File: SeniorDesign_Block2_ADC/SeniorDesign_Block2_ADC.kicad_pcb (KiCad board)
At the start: 2 copper layers, 40 x 75 mm, 18 parts, among them J1 Conn_02x18_Row_Letter_First, J2 Conn_02x18_Row_Letter_First, U1 AD9283, X1 ASE-xxxMHz

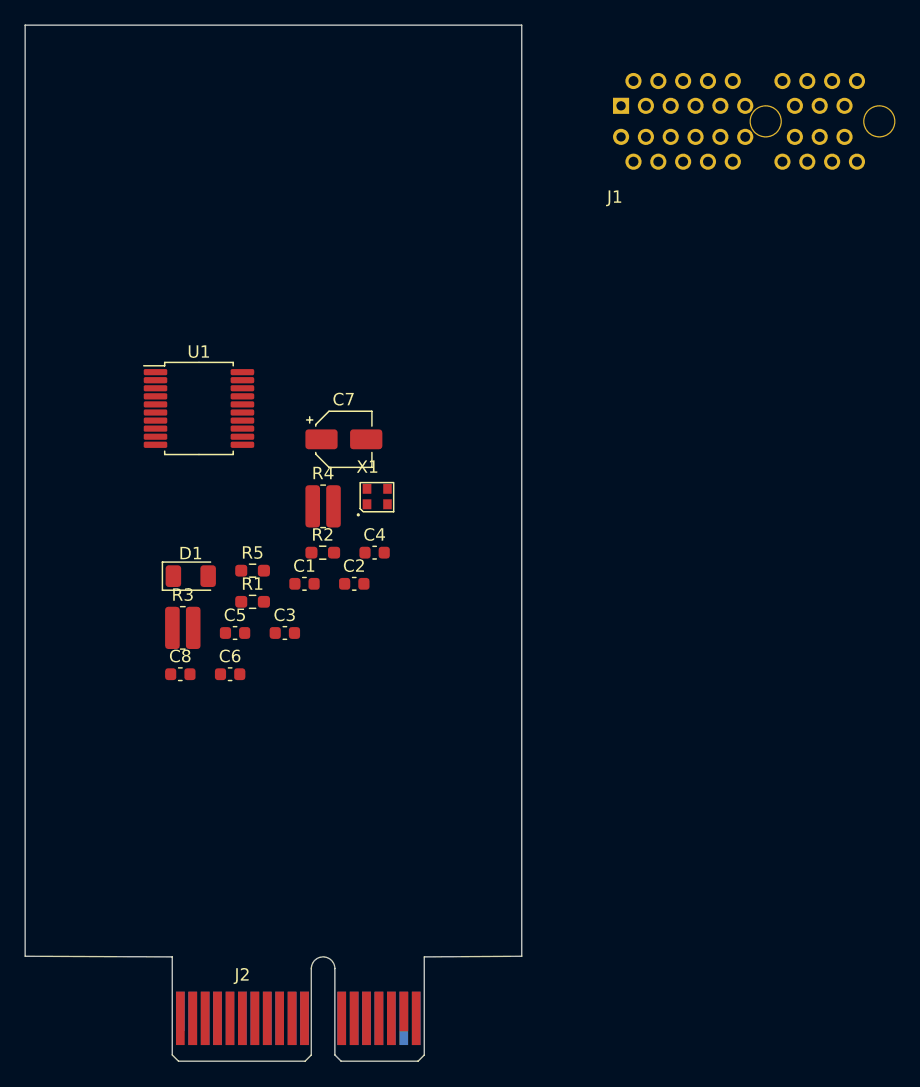
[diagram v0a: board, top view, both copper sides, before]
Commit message: Continued work.  Push to github.  Even worse commit messages.
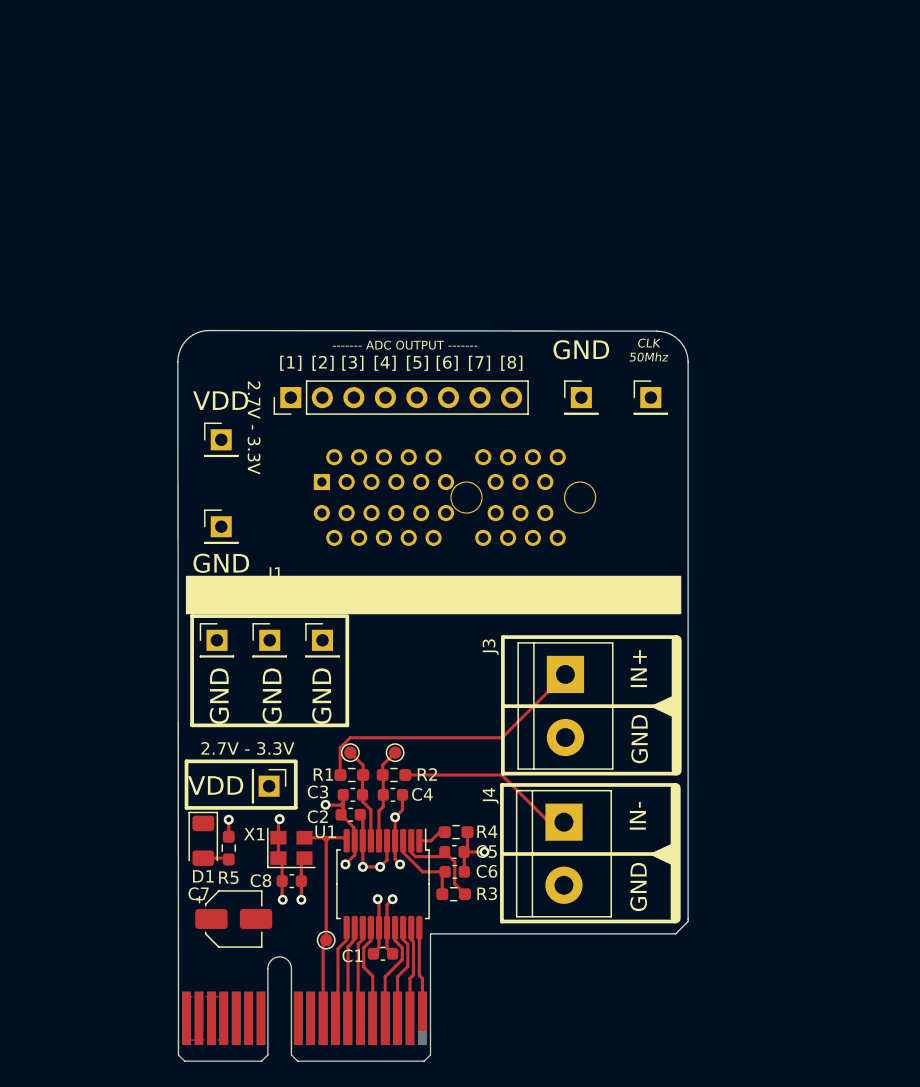
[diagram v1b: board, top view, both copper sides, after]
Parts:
- added J10: Conn_01x01, Connector_PinHeader_2.54mm:PinHeader_1x01_P2.54mm_Vertical, F.Cu at (145.4, 55.0)
- added J11: Conn_01x08, Connector_PinHeader_2.54mm:PinHeader_1x08_P2.54mm_Vertical, F.Cu at (116.4, 55.0)
- added J12: Conn_01x01, Connector_PinHeader_2.54mm:PinHeader_1x01_P2.54mm_Vertical, F.Cu at (110.8, 58.4)
- added J13: Conn_01x01, Connector_PinHeader_2.54mm:PinHeader_1x01_P2.54mm_Vertical, F.Cu at (139.8, 55.0)
- added J3: Conn_01x02_Male, TerminalBlock:TerminalBlock_bornier-2_P5.08mm, F.Cu at (138.5, 77.3)
- added J4: Conn_01x02_Male, TerminalBlock:TerminalBlock_bornier-2_P5.08mm, F.Cu at (138.4, 89.2)
- added J5: Conn_01x01, Connector_PinHeader_2.54mm:PinHeader_1x01_P2.54mm_Vertical, F.Cu at (114.7, 74.5)
- added J6: Conn_01x01, Connector_PinHeader_2.54mm:PinHeader_1x01_P2.54mm_Vertical, F.Cu at (110.5, 74.5)
- added J7: Conn_01x01, Connector_PinHeader_2.54mm:PinHeader_1x01_P2.54mm_Vertical, F.Cu at (119.0, 74.5)
- added J8: Conn_01x01, Connector_PinHeader_2.54mm:PinHeader_1x01_P2.54mm_Vertical, F.Cu at (114.7, 86.3)
- added J9: Conn_01x01, Connector_PinHeader_2.54mm:PinHeader_1x01_P2.54mm_Vertical, F.Cu at (110.8, 65.4)
- added TP1: TestPoint_Small, TestPoint:TestPoint_Pad_D1.0mm, F.Cu at (121.2, 83.6)
- added TP2: TestPoint_Small, TestPoint:TestPoint_Pad_D1.0mm, F.Cu at (124.8, 83.6)
- added TP4: TestPoint_Small, TestPoint:TestPoint_Pad_D1.0mm, F.Cu at (119.2, 98.7)
- J2: moved to B.Cu
- R3, R4: footprint Resistor_SMD:R_0612_1632Metric_Pad1.18x3.40mm_HandSolder -> Resistor_SMD:R_0603_1608Metric_Pad0.98x0.95mm_HandSolder
- X1: footprint SeniorDesign_Block2_ADC:DSC6001JI1A_Oscillator -> Oscillator:Oscillator_SMD_Abracon_ASE-4Pin_3.2x2.5mm
- moved U1 41.1 mm to (123.8, 94.2), turned to 270 degrees
- moved C7 39.6 mm to (111.8, 97.0)
- moved J1 38.7 mm to (130.9, 62.8)
- moved R3 30.6 mm to (129.5, 95.0)
- moved C1 30.5 mm to (123.8, 99.8)
- moved R4 28.3 mm to (129.7, 90.0)
- moved X1 28.3 mm to (116.5, 91.3)
- moved C5 25.0 mm to (129.6, 91.6)
- moved C6 24.1 mm to (129.6, 93.2)
- moved R5 22.4 mm to (111.4, 91.3), turned to 270 degrees
- moved D1 21.3 mm to (109.3, 90.7), turned to 270 degrees
- moved C4 19.6 mm to (124.6, 87.0)
- moved J2 19.5 mm to (127.0, 105.0), turned to 180 degrees
- moved C8 18.9 mm to (116.5, 94.0)
- moved R2 18.8 mm to (124.7, 85.4)
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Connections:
- J1 pad A1: (no net) -> /conn_adc_a1
- J1 pad A10: (no net) -> conn_gnd
- J1 pad A11: (no net) -> conn_gnd
- J1 pad A12: (no net) -> conn_gnd
- J1 pad A13: (no net) -> conn_gnd
- J1 pad A14: (no net) -> conn_gnd
- J1 pad A15: (no net) -> conn_vdd
- J1 pad A16: (no net) -> conn_vdd
- J1 pad A17: (no net) -> conn_vdd
- J1 pad A18: (no net) -> conn_vdd
- J1 pad A2: (no net) -> /conn_adc_a2
- J1 pad A3: (no net) -> /conn_adc_a3
- J1 pad A4: (no net) -> /conn_adc_a4
- J1 pad A5: (no net) -> /conn_adc_a5
- J1 pad A6: (no net) -> /conn_adc_a6
- J1 pad A7: (no net) -> /conn_adc_a7
- J1 pad A8: (no net) -> /conn_adc_a8
- J1 pad A9: (no net) -> conn_clk
- J1 pad B1: (no net) -> conn_gnd
- J1 pad B10: (no net) -> conn_gnd
- J1 pad B11: (no net) -> conn_gnd
- J1 pad B12: (no net) -> conn_gnd
- J1 pad B13: (no net) -> conn_gnd
- J1 pad B14: (no net) -> conn_gnd
- J1 pad B15: (no net) -> conn_gnd
- J1 pad B16: (no net) -> conn_gnd
- J1 pad B17: (no net) -> conn_gnd
- J1 pad B18: (no net) -> conn_gnd
- J1 pad B2: (no net) -> conn_gnd
- J1 pad B3: (no net) -> conn_gnd
- J1 pad B4: (no net) -> conn_gnd
- J1 pad B5: (no net) -> conn_gnd
- J1 pad B6: (no net) -> conn_gnd
- J1 pad B7: (no net) -> conn_gnd
- J1 pad B8: (no net) -> conn_gnd
- J1 pad B9: (no net) -> conn_gnd
- J2 pad A1: (no net) -> /adc_a1
- J2 pad A10: (no net) -> /gnd
- J2 pad A11: (no net) -> /gnd
- J2 pad A12: (no net) -> /gnd
- J2 pad A13: (no net) -> /gnd
- J2 pad A14: (no net) -> /gnd
- J2 pad A15: (no net) -> vdd
- J2 pad A16: (no net) -> vdd
- J2 pad A17: (no net) -> vdd
- J2 pad A18: (no net) -> vdd
- J2 pad A2: (no net) -> /adc_a2
- J2 pad A3: (no net) -> /adc_a3
- J2 pad A4: (no net) -> /adc_a4
- J2 pad A5: (no net) -> /adc_a5
- J2 pad A6: (no net) -> /adc_a6
- J2 pad A7: (no net) -> /adc_a7
- J2 pad A8: (no net) -> /adc_a8
- J2 pad A9: (no net) -> clk
- J2 pad B1: (no net) -> /gnd
- J2 pad B10: (no net) -> /gnd
- J2 pad B11: (no net) -> /gnd
- J2 pad B12: (no net) -> /gnd
- J2 pad B13: (no net) -> /gnd
- J2 pad B14: (no net) -> /gnd
- J2 pad B15: (no net) -> /gnd
- J2 pad B16: (no net) -> /gnd
- J2 pad B17: (no net) -> /gnd
- J2 pad B18: (no net) -> /gnd
- J2 pad B2: (no net) -> /gnd
- J2 pad B3: (no net) -> /gnd
- J2 pad B4: (no net) -> /gnd
- J2 pad B5: (no net) -> /gnd
- J2 pad B6: (no net) -> /gnd
- J2 pad B7: (no net) -> /gnd
- J2 pad B8: (no net) -> /gnd
- J2 pad B9: (no net) -> /gnd
- R1 pad 2: (no net) -> in_a+
- R2 pad 2: (no net) -> in_a-
- U1 pad 11: (no net) -> /adc_a8
- U1 pad 12: (no net) -> /adc_a7
- U1 pad 13: (no net) -> /adc_a6
- U1 pad 14: (no net) -> /adc_a5
- U1 pad 17: (no net) -> /adc_a4
- U1 pad 18: (no net) -> /adc_a3
- U1 pad 19: (no net) -> /adc_a2
- U1 pad 20: (no net) -> /adc_a1
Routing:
- net GND: track 0.00 -> 27.7 mm, vias 0 -> 7
- net in_a+: track 0.00 -> 22.8 mm
- net vdd: track 0.00 -> 20.7 mm, vias 0 -> 6
- net clk: track 0.00 -> 19.1 mm
- net in_a-: track 0.00 -> 14.3 mm
- net /adc_a4: track 0.00 -> 8.11 mm
- net Net-(C5-Pad1): track 0.00 -> 8.01 mm
- net /adc_a5: track 0.00 -> 7.84 mm
- net Net-(C3-Pad1): track 0.00 -> 7.82 mm
- net /adc_a3: track 0.00 -> 7.80 mm
- net Net-(C4-Pad1): track 0.00 -> 7.68 mm
- net /adc_a8: track 0.00 -> 7.67 mm
- net /adc_a6: track 0.00 -> 7.53 mm
- net /adc_a7: track 0.00 -> 7.53 mm
- net /adc_a2: track 0.00 -> 7.49 mm
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- added copper zone on In1.Cu, net GND
- added copper zone on In1.Cu, net conn_gnd
- added copper zone on In2.Cu, net conn_vdd
- added copper zone on F.Cu, net vdd
- added copper zone on In2.Cu, net vdd
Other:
- board size 40 x 75 mm -> 41.1 x 50.4 mm
- copper layers 2 -> 4
- board text added: "------- ADC OUTPUT -------"
- board text added: "2.7V - 3.3V"
- board text added: "CLK 50Mhz"
- board text added: "GND"
- board text added: "IN+"
- board text added: "IN-"
- board text added: "VDD"
- board text added: "[1]"
- board text added: "[2]"
- board text added: "[3]"
- board text added: "[4]"
- board text added: "[5]"
- board text added: "[6]"
- board text added: "[7]"
- board text added: "[8]"
